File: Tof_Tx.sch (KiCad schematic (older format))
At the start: 74 parts, among them M1 mounting_holes_laser, M2 mounting_holes_laser, U10 NC7WZ00K8X, U11 UMCC_50Ohm, U12 UMCC_50Ohm, U13 NC7WZ00K8X, U14 NCP81074BDR2G, U34 NC7WZ16, U4 UMCC_50Ohm, U5 UMCC_50Ohm, U6 HMC589AST89E, U7 TLV3501, U8 UMCC_50Ohm, U9 NC7WZ00K8X

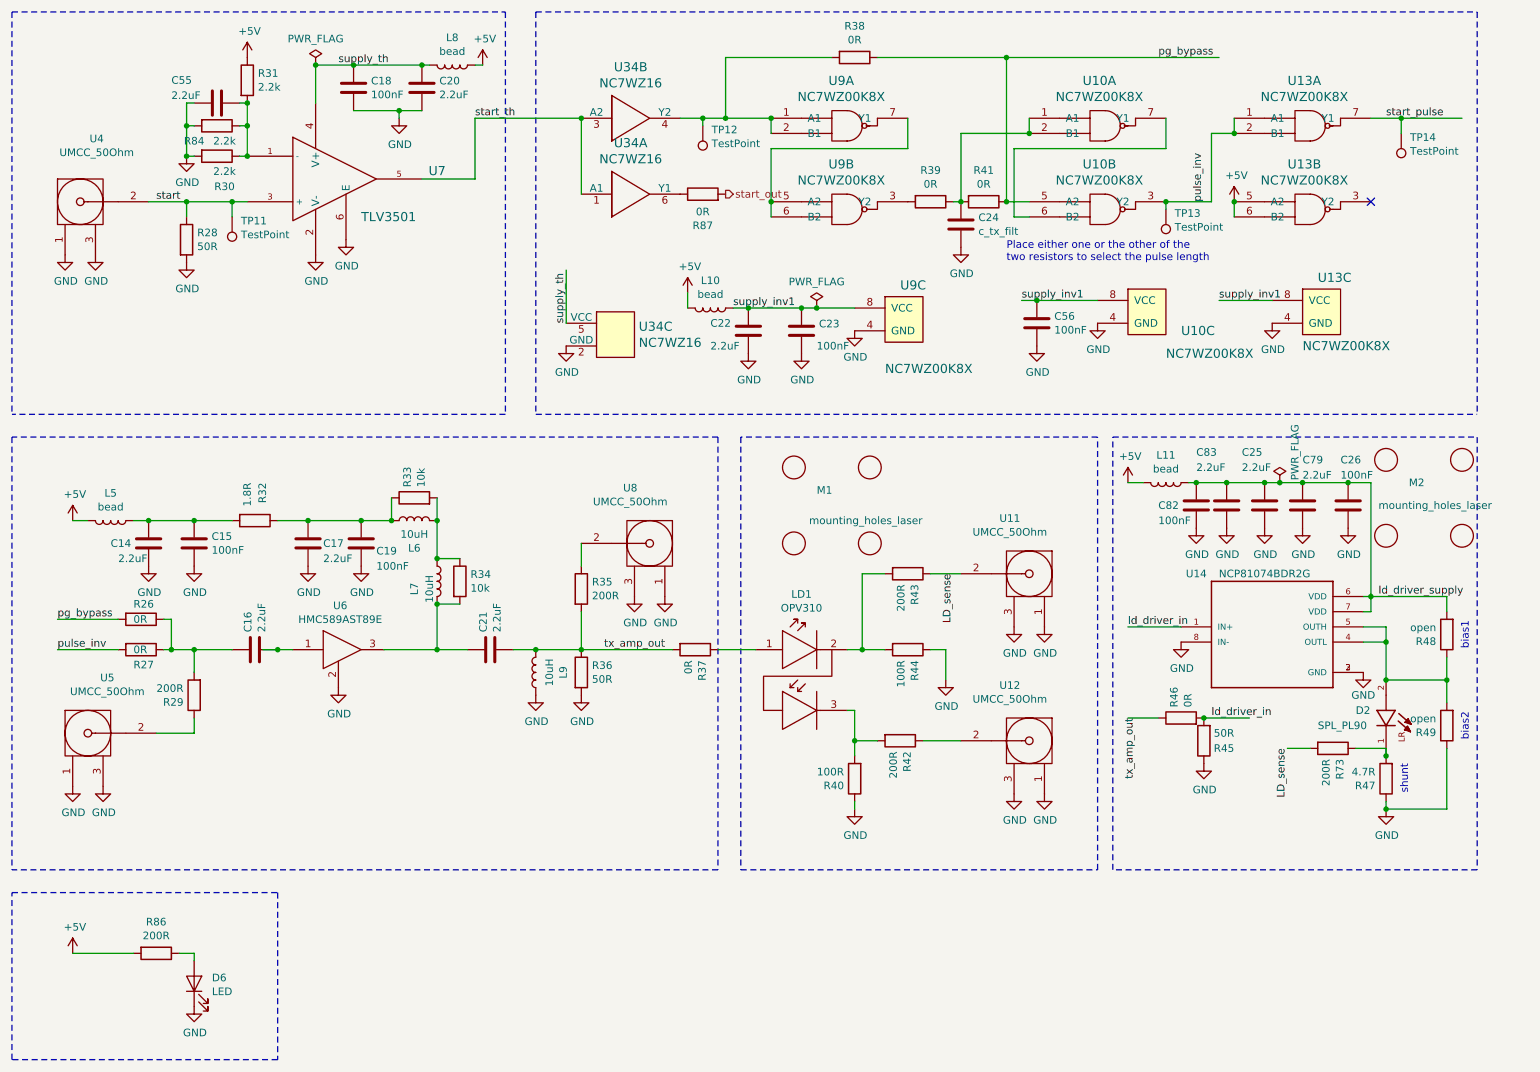
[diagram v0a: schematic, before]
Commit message: Version 1.0. As ordered at PCBWay on 13.11.2019
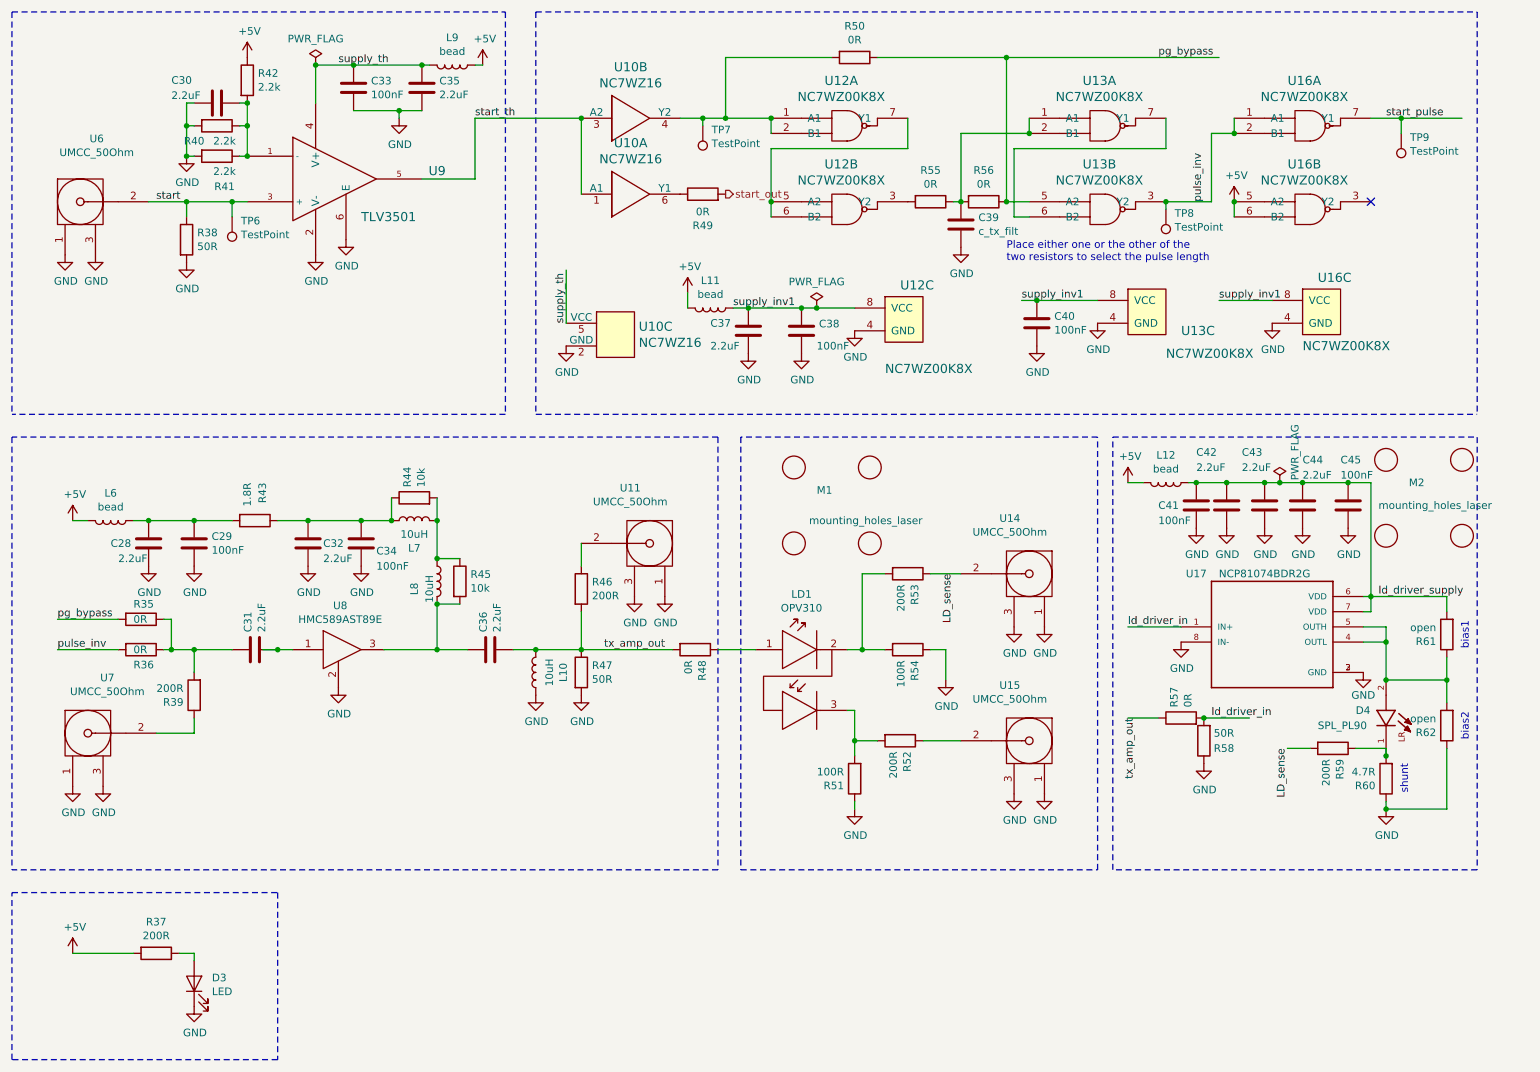
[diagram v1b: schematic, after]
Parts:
- renumbered C14 to C28, C15 to C29, C55 to C30, C16 to C31, C17 to C32, C18 to C33, C19 to C34, C20 to C35, C21 to C36, C22 to C37, C23 to C38, C24 to C39, C56 to C40, C82 to C41, C83 to C42, C25 to C43, C79 to C44, C26 to C45, D6 to D3, D2 to D4, L9 to L10, L10 to L11, L11 to L12, L5 to L6, L6 to L7, L7 to L8, L8 to L9, R26 to R35, R27 to R36, R86 to R37, R28 to R38, R29 to R39, R84 to R40, R30 to R41, R31 to R42, R32 to R43, R33 to R44, R34 to R45, R35 to R46, R36 to R47, R37 to R48, R87 to R49, R38 to R50, R40 to R51, R42 to R52, R43 to R53, R44 to R54, R39 to R55, R41 to R56, R46 to R57, R45 to R58, R73 to R59, R47 to R60, R48 to R61, R49 to R62, TP11 to TP6, TP12 to TP7, TP13 to TP8, TP14 to TP9, U34 to U10, U8 to U11, U9 to U12, U10 to U13, U11 to U14, U12 to U15, U13 to U16, U14 to U17, U4 to U6, U5 to U7, U6 to U8, U7 to U9
